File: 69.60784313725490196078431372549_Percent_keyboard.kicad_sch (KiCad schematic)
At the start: 5 parts, among them U1 ATMEGA32U4-AU

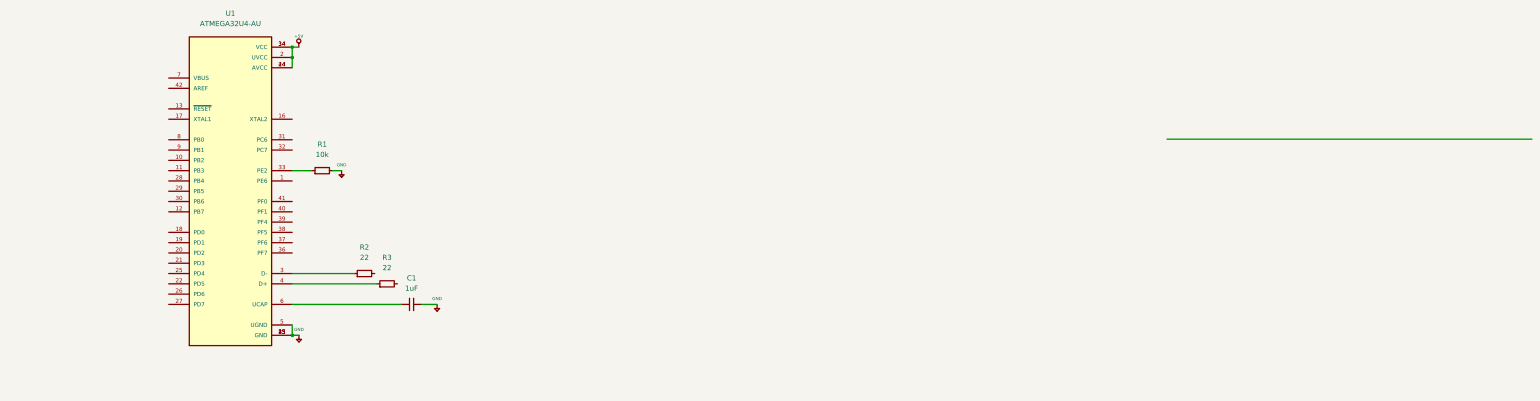
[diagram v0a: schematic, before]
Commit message: reset push button, crystal
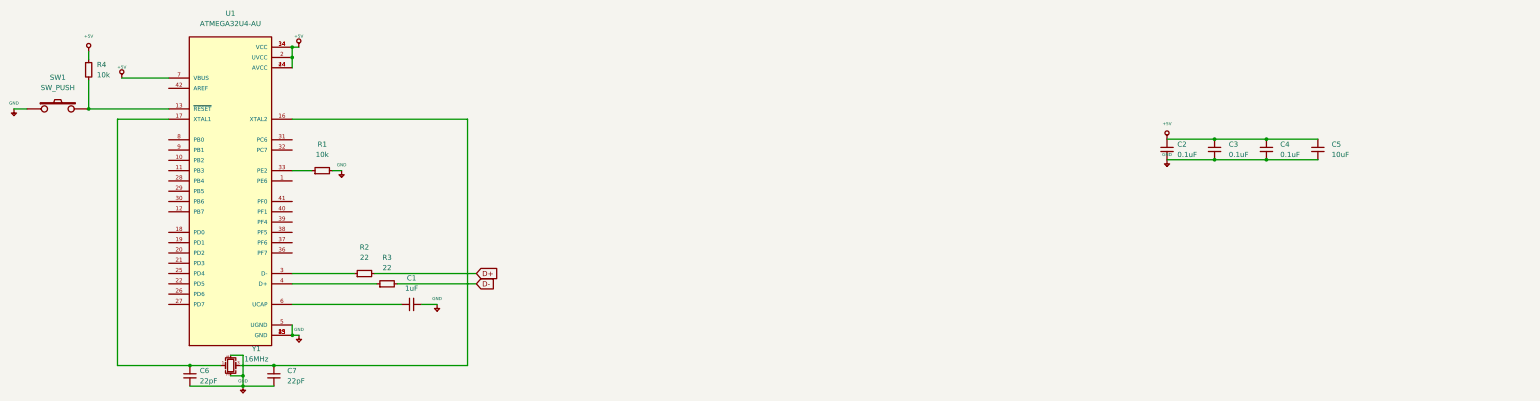
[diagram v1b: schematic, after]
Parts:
- added C2, C3, C4: 0.1uF, symbol Device:C_Small
- added C5: 10uF, symbol Device:C_Small
- added C6, C7: 22pF, symbol Device:C_Small
- added R4: 10k, symbol Device:R_Small
- added SW1: SW_PUSH, symbol keyboard_parts:SW_PUSH
- added Y1: 16MHz, symbol Device:Crystal_GND24_Small
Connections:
- net +5V: now also U1.7 (VBUS), C2.1, C2.2, C3.1, C3.2, C4.1, C4.2, C5.1, C5.2, C6.2, C7.2, R4.1, SW1.1, Y1.2, Y1.4
- net D+: now reaches R2.2
- net D-: now reaches R3.2
- net at U1.13 (~{RESET}): now also R4.2, SW1.2
- net at U1.16 (XTAL2): now also C7.1, Y1.3
- net at U1.17 (XTAL1): now also C6.1, Y1.1
